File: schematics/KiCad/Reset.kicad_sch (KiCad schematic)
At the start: 12 parts, among them SW2 RESET, SW3 RESET, U11 74HC08, U14 DS1232, U15 74HC132

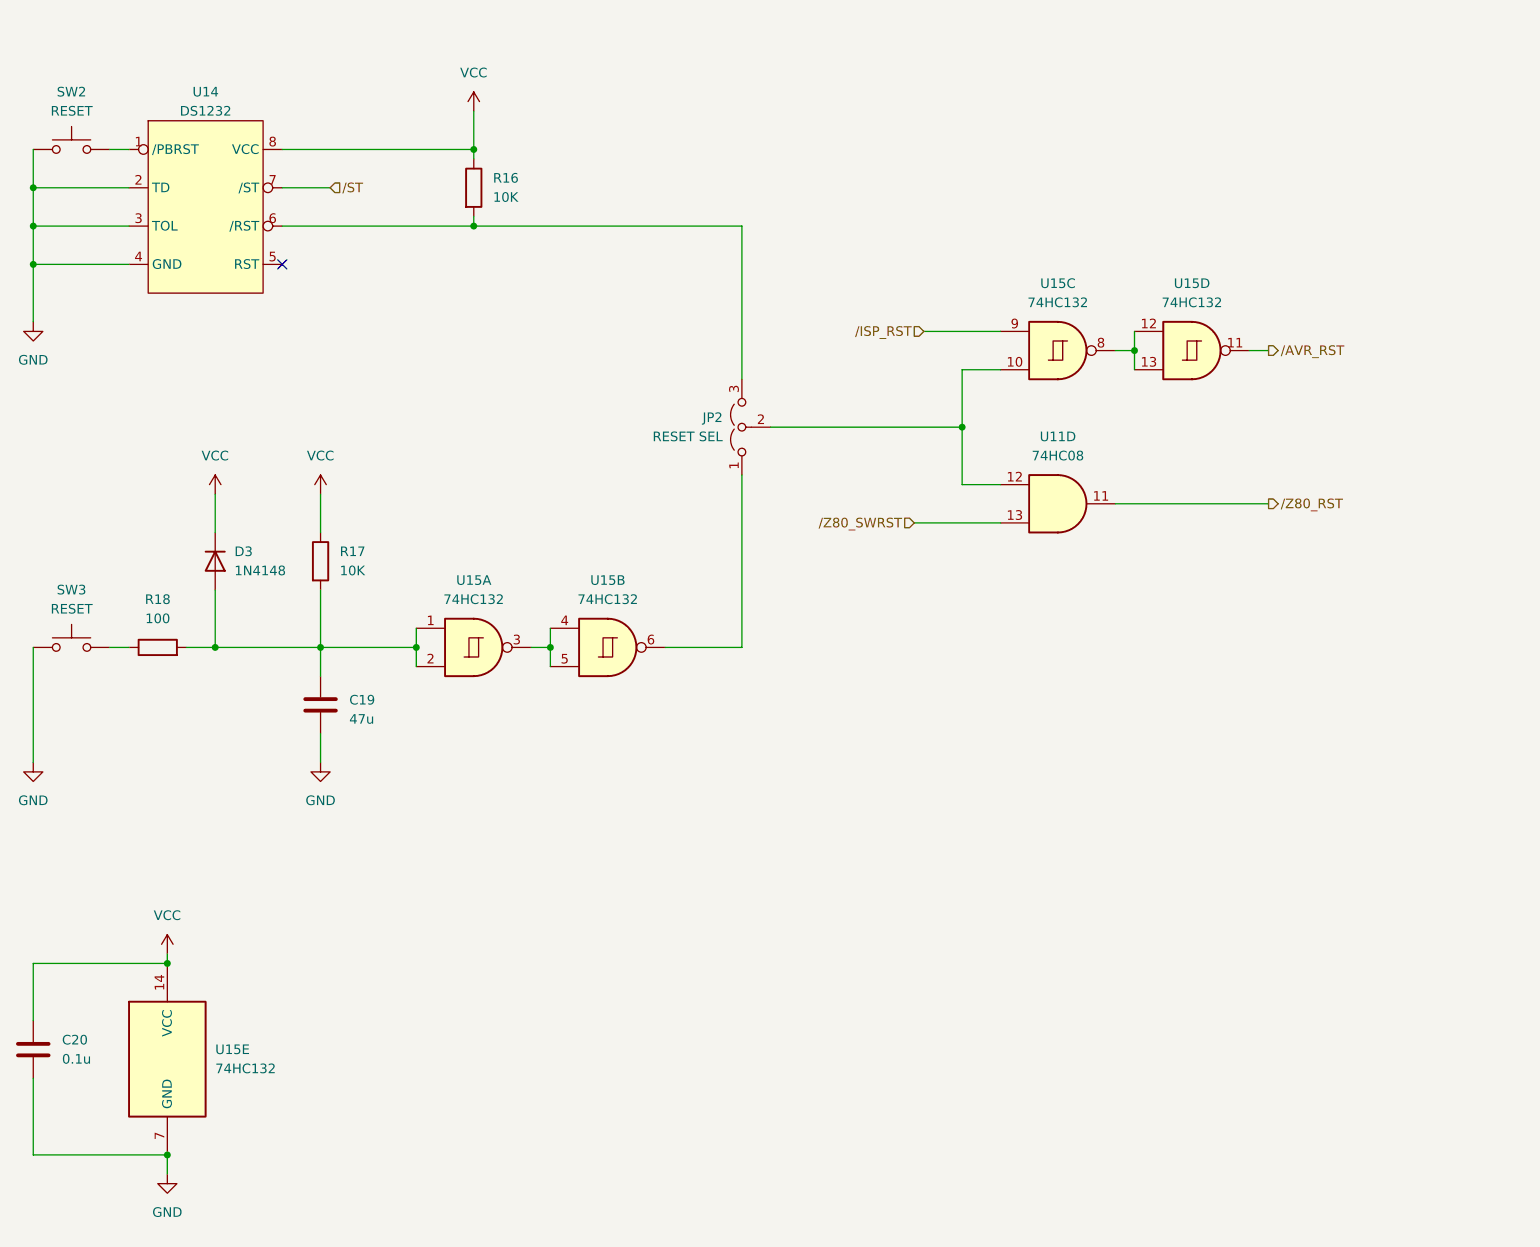
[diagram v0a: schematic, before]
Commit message: Update schematics.
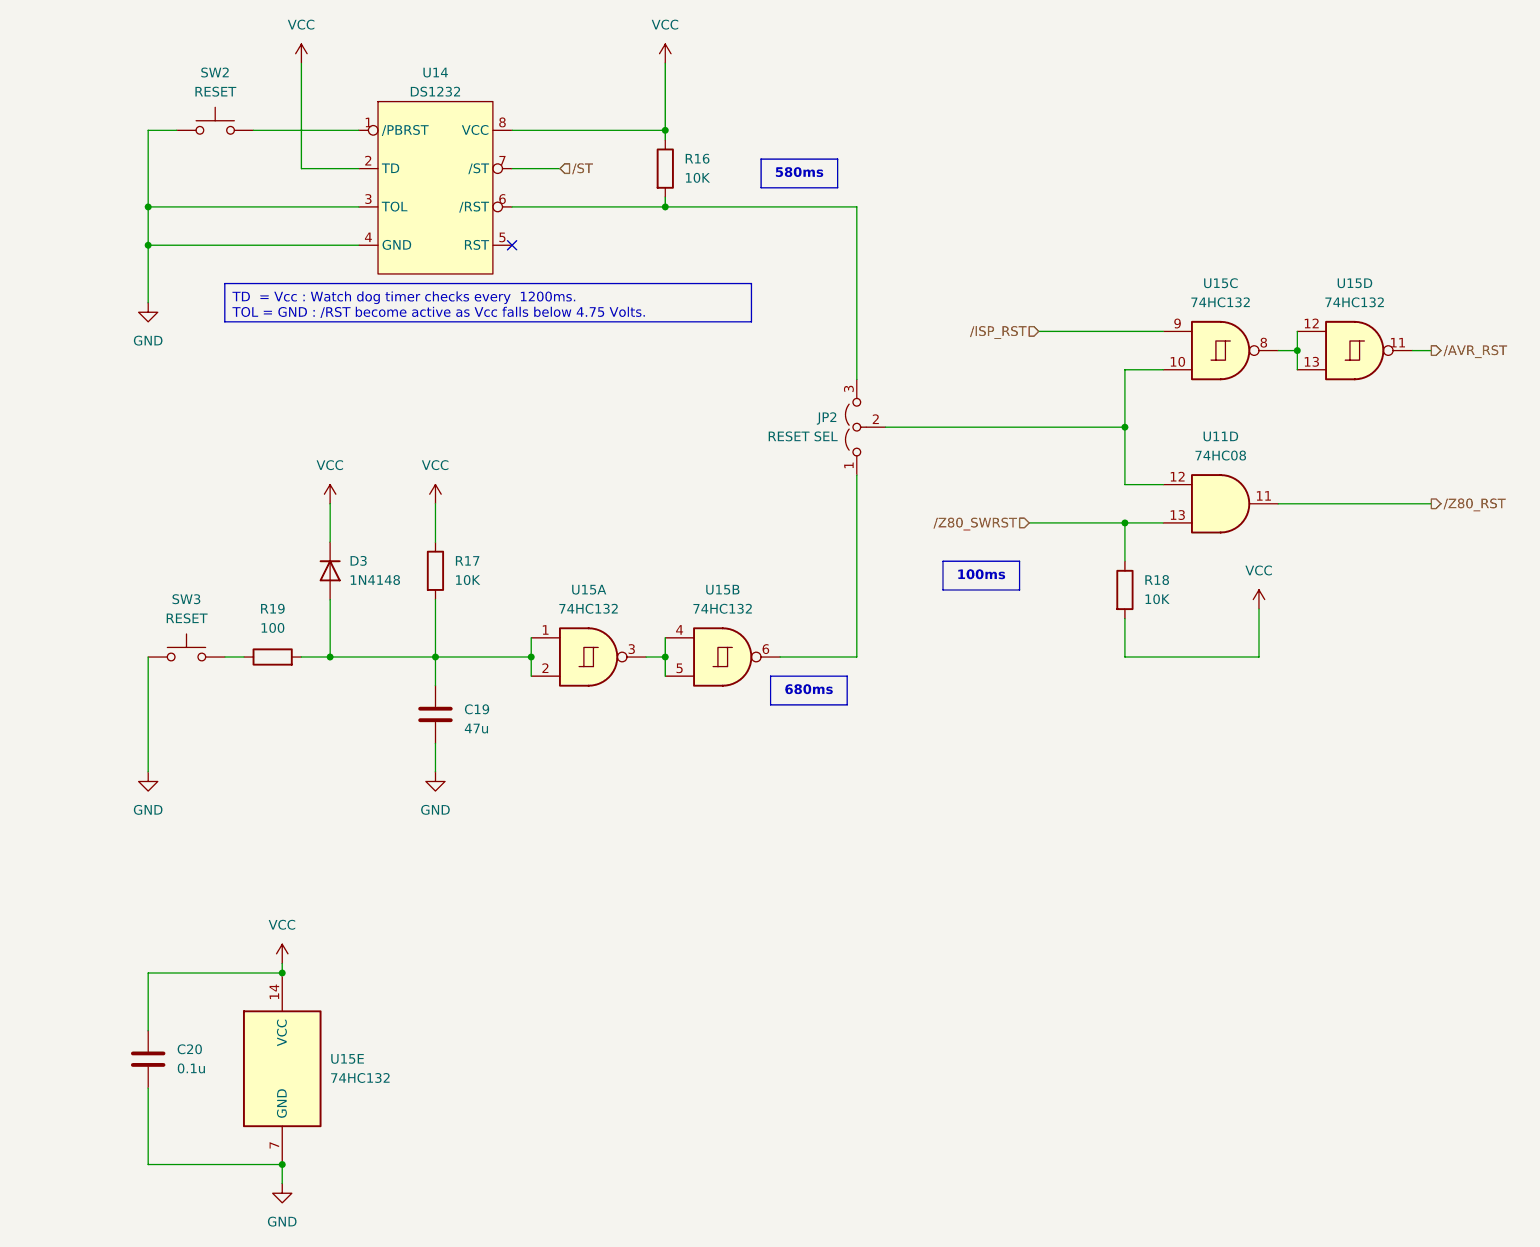
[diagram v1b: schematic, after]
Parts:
- added R18: 10K, Resistor_THT:R_Axial_DIN0204_L3.6mm_D1.6mm_P7.62mm_Horizontal, symbol Device:R
- renumbered R18 to R19
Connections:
- net GND: no longer U14.2 (TD)
- net VCC: now also U14.2 (TD), R18.2
- net /Z80_SWRST: now also R18.1
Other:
- company: (none) -> By 46nori
- moved on the sheet: C19, C20, D3, JP2, R16, R17, R19, SW2, SW3, U11D, U14, U15A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
